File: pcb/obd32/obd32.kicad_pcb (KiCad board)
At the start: 2 copper layers, 43.2 x 43.2 mm, 36 parts, among them J1 USB_C_Receptacle_USB2.0, J2 Micro_SD_Card, J3 Conn_02x08_Top_Bottom, J4 USB_A, U1 LMR33630ADDA, U2 CP2102N-A01-GQFN24, U3 AP1117-33, U4 ESP32-WROOM-32, U5 SiP32431DR3, U6 MCP2562-E-MF

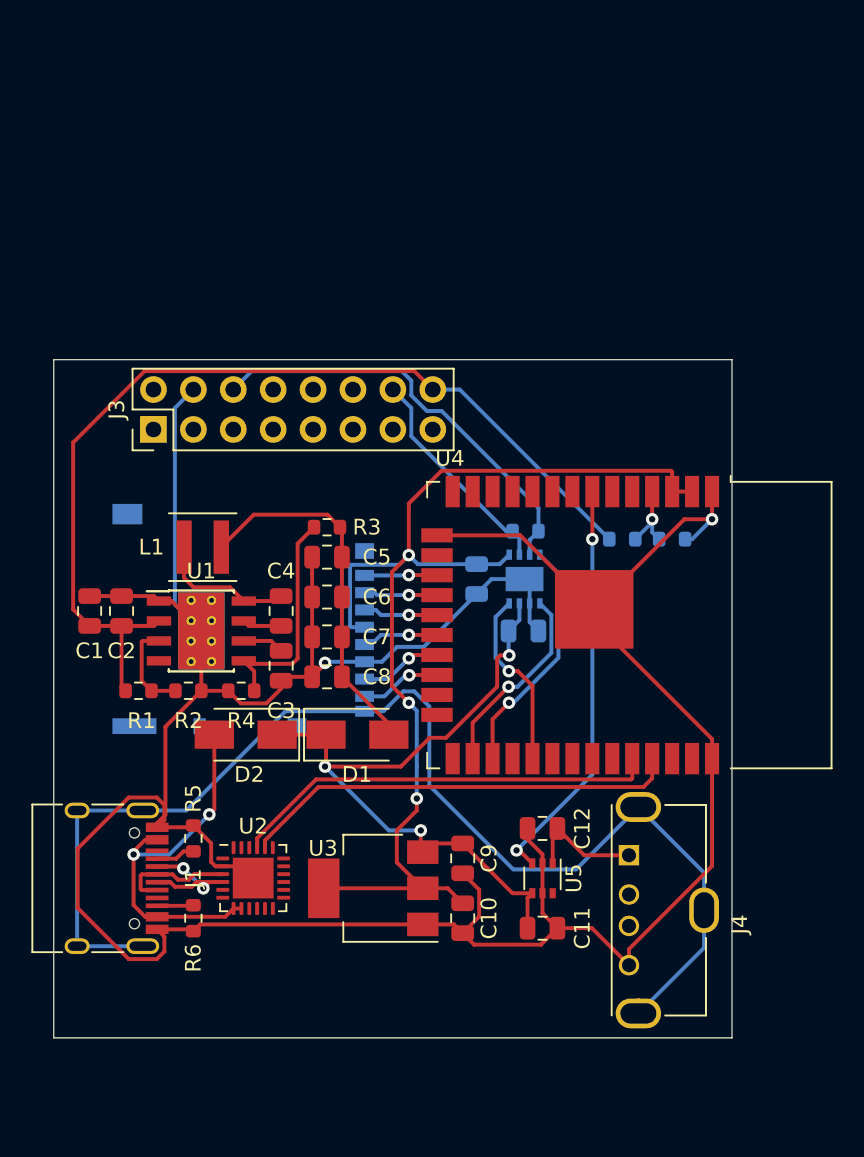
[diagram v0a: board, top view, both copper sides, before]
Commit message: Maybe version of board
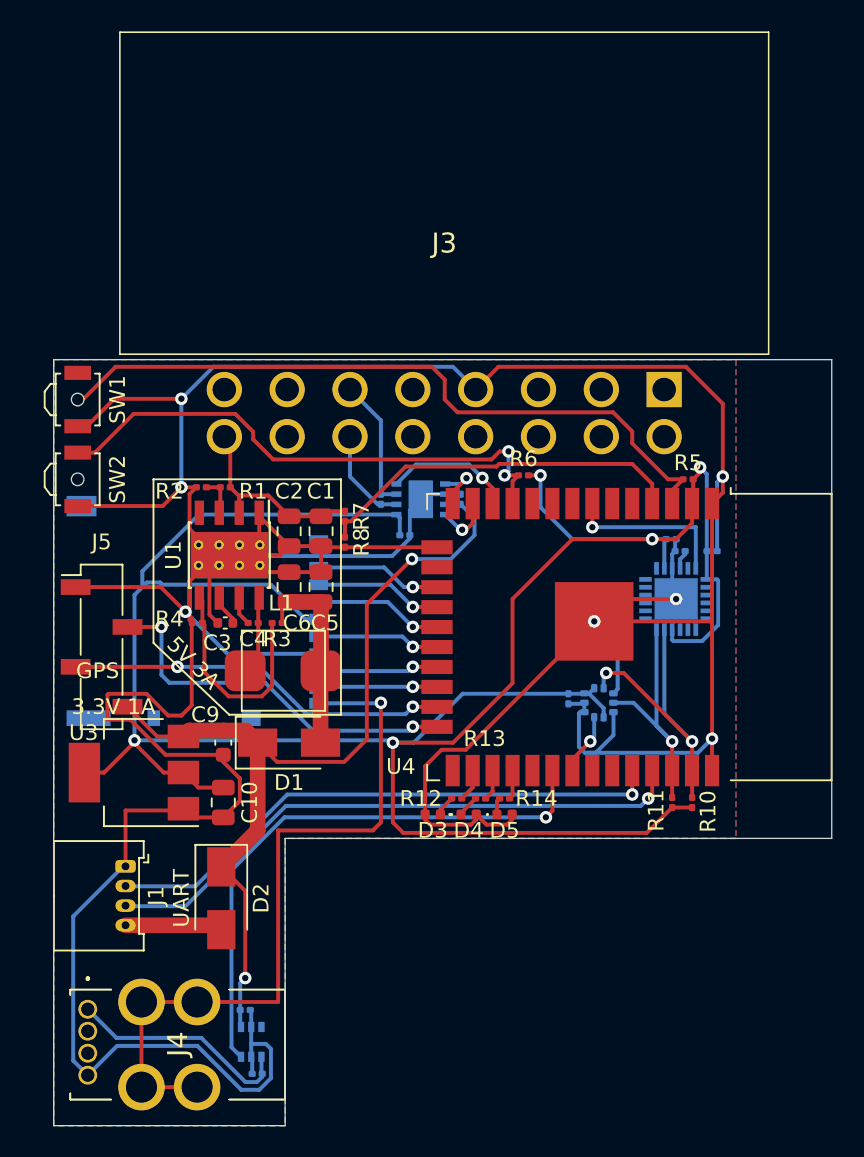
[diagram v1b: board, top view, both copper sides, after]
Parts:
- removed C7, C8: 22µF, Capacitor_SMD:C_0805_2012Metric
- added C15: 10nF, Capacitor_SMD:C_0201_0603Metric, B.Cu at (236.2, 73.7)
- added C16: 0.47µF, Capacitor_SMD:C_0201_0603Metric, B.Cu at (236.7, 74.4)
- added C17: 0.1µF, Capacitor_SMD:C_0201_0603Metric, B.Cu at (238.8, 74.4)
- added C18: 0.1µF, Capacitor_SMD:C_0201_0603Metric, B.Cu at (229.6, 83.8)
- added D3: LED, LED_SMD:LED_0402_1005Metric, F.Cu at (221.0, 91.2)
- added D4: LED, LED_SMD:LED_0402_1005Metric, F.Cu at (223.3, 91.2)
- added D5: LED, LED_SMD:LED_0402_1005Metric, F.Cu at (225.6, 91.2)
- added J5: Conn_01x04_Female, Connector_PinSocket_2.54mm:PinSocket_1x04_P2.54mm_Vertical_SMD_Pin1Left, F.Cu at (199.9, 80.5)
- added R10: 4K7, Resistor_SMD:R_0201_0603Metric, F.Cu at (236.2, 90.4)
- added R11: 4K7, Resistor_SMD:R_0201_0603Metric, F.Cu at (237.5, 90.4)
- added R12: 65R, Resistor_SMD:R_0201_0603Metric, F.Cu at (222.5, 90.2)
- added R13: 65R, Resistor_SMD:R_0201_0603Metric, F.Cu at (224.0, 90.2)
- added R14: 5R, Resistor_SMD:R_0201_0603Metric, F.Cu at (225.6, 90.2)
- added SW1: SW_Push, Button_Switch_SMD:SW_SPST_B3U-3000P-B, F.Cu at (198.4, 64.8)
- added SW2: SW_Push, Button_Switch_SMD:SW_SPST_B3U-3000P-B, F.Cu at (198.4, 69.8)
- added U7: LPS25HB, Package_LGA:ST_HLGA-10_2.5x2.5mm_P0.6mm_LayoutBorder3x2y, B.Cu at (231.6, 84.1)
- C11, C12: value 100nF -> 0.1µF; footprint Capacitor_SMD:C_0805_2012Metric -> Capacitor_SMD:C_0201_0603Metric; moved to B.Cu
- C13, C14, C4: value 100nF -> 0.1µF; footprint Capacitor_SMD:C_0805_2012Metric -> Capacitor_SMD:C_0201_0603Metric
- C3: footprint Capacitor_SMD:C_0805_2012Metric -> Capacitor_SMD:C_0402_1005Metric
- C9: footprint Capacitor_SMD:C_0805_2012Metric -> Capacitor_SMD:C_0603_1608Metric
- J1: value USB_C_Receptacle_USB2.0 -> Conn_01x04_Male; footprint Connector_USB:USB_C_Receptacle_HRO_TYPE-C-31-M-12 -> Connector_Molex:Molex_PicoBlade_53048-0410_1x04_P1.25mm_Horizontal
- J3: value Conn_02x08_Top_Bottom -> OBD2; footprint Connector_PinHeader_2.54mm:PinHeader_2x08_P2.54mm_Vertical -> OBD2:OBD2
- J4: value USB_A -> 67329-8040; footprint Connector_USB:USB_A_Molex_105057_Vertical -> 67329-8040:673298040
- L1: value 8µH -> 2.2µH; footprint Inductor_SMD:L_Coilcraft_XxL4040 -> TDK_SPM5030:TDK_SPM5030
- R1, R2, R3, R4, R9: footprint Resistor_SMD:R_0603_1608Metric -> Resistor_SMD:R_0201_0603Metric
- R5, R6: value 5K1 -> 100K; footprint Resistor_SMD:R_0603_1608Metric -> Resistor_SMD:R_0201_0603Metric
- R7, R8: footprint Resistor_SMD:R_0603_1608Metric -> Resistor_SMD:R_0201_0603Metric; moved to F.Cu
- U1: value LMR33630ADDA -> LMR33630BDDA
- U2: value CP2102N-A01-GQFN24 -> ICM-20689; footprint Package_DFN_QFN:QFN-24-1EP_4x4mm_P0.5mm_EP2.6x2.6mm -> ICM-20689:QFN50P400X400X95-25N-D; moved to B.Cu
- U5: moved to B.Cu
- moved R5 38.9 mm to (237.2, 69.8), turned to 0 degrees
- moved J4 35.8 mm to (199.0, 103.6), turned to 90 degrees
- moved R6 35.2 mm to (226.8, 69.6), turned to 0 degrees
- moved J3 32.6 mm to (235.7, 64.1), turned to 180 degrees
- moved U2 32.3 mm to (236.5, 77.5)
- moved C12 24.0 mm to (209.8, 107.7)
- moved U5 21.3 mm to (209.4, 105.7), turned to 90 degrees
- moved R8 20.8 mm to (215.4, 73.8), turned to 270 degrees
- moved C11 19.6 mm to (209.0, 103.6)
- moved R7 17.7 mm to (215.4, 72.2), turned to 270 degrees
- moved C10 16.9 mm to (207.6, 90.4)
- moved C9 16.9 mm to (207.6, 86.6)
- moved U3 16.9 mm to (202.0, 88.5)
- moved C1 15.6 mm to (213.9, 73.2), turned to 270 degrees
- moved R1 14.1 mm to (207.8, 70.4), turned to 180 degrees
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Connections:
- J2 pad 9: Earth -> GND
- R5 pad 1: GND -> ESP32_EN
- R5 pad 2: Net-(J1-PadA5) -> +3V3
- R6 pad 1: Net-(J1-PadB5) -> ESP32_MISC
- R6 pad 2: GND -> +3V3
- U2 pad 10: (no net) -> Net-(C16-Pad2)
- U2 pad 12: (no net) -> IMU_INT
- U2 pad 13: (no net) -> +3V3
- U2 pad 2: GND -> (no net)
- U2 pad 20: UART_TX -> (no net)
- U2 pad 21: UART_RX -> (no net)
- U2 pad 22: (no net) -> +3V3
- U2 pad 23: (no net) -> I2C0_SCL
- U2 pad 24: (no net) -> I2C0_SDA
- U2 pad 3: USB_D+ -> (no net)
- U2 pad 4: USB_D- -> (no net)
- U2 pad 7: +5VA -> (no net)
- U2 pad 8: +5VA -> +3V3
- U2 pad 9: (no net) -> GND
- U4 pad 11: (no net) -> ESP32_MISC
- U4 pad 12: (no net) -> CAN_SHDN
- U4 pad 13: (no net) -> CAN_RX
- U4 pad 14: (no net) -> CAN_TX
- U4 pad 23: (no net) -> GPS_RX
- U4 pad 24: (no net) -> GPS_TX
- U4 pad 26: CAN_TX -> LED_R
- U4 pad 27: CAN_SHDN -> LED_G
- U4 pad 28: (no net) -> LED_B
- U4 pad 29: CAN_RX -> (no net)
- U4 pad 3: +3V3 -> ESP32_EN
- U4 pad 30: (no net) -> USB_EN
- U4 pad 31: (no net) -> BARO_INT
- U4 pad 36: (no net) -> I2C0_SDA
- U4 pad 37: (no net) -> I2C0_SCL
- U4 pad 7: USB_EN -> IMU_INT
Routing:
- net GND: track 203.4 -> 351.0 mm, vias 2 -> 8
- net +3V3: track 71.9 -> 171.7 mm, vias 3 -> 5
- net Earth: track 78.5 -> 0.00 mm
- net +BATT: track 61.8 -> 13.7 mm
- net ESP32_EN: track 0.00 -> 45.5 mm
- net ESP32_MISC: track 0.00 -> 34.6 mm, vias 0 -> 2
- net GPS_RX: track 0.00 -> 24.4 mm, vias 0 -> 2
- net GPS_TX: track 0.00 -> 24.3 mm, vias 0 -> 2
- net I2C0_SCL: track 0.00 -> 19.7 mm, vias 0 -> 2
- net Net-(R7-Pad2): track 4.93 -> 23.9 mm, vias 1 -> 0
- net CAN_H: track 27.3 -> 8.47 mm
- net +5VA: track 23.7 -> 6.21 mm, vias 2 -> 0
- net I2C0_SDA: track 0.00 -> 15.9 mm, vias 0 -> 1
- net +5V: track 44.6 -> 58.0 mm, vias 3 -> 2
- net Net-(C5-Pad1): track 23.2 -> 12.5 mm
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- added copper zone on B.Cu, net GND
- added copper zone on F.Cu, net GND
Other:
- board size 43.2 x 43.2 mm -> 49.5 x 48.8 mm
- board text added: "5V 3A"
- board text added: "GPS"
- board text added: "UART"
- board text removed: "5V 3A DC-DC"
